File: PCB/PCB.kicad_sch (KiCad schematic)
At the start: 17 parts, among them J1 Conn_01x06_Pin, U2 A7106, U3 HT7333-3.3V, U4 STM32G031F6Px, Y1 16MHz

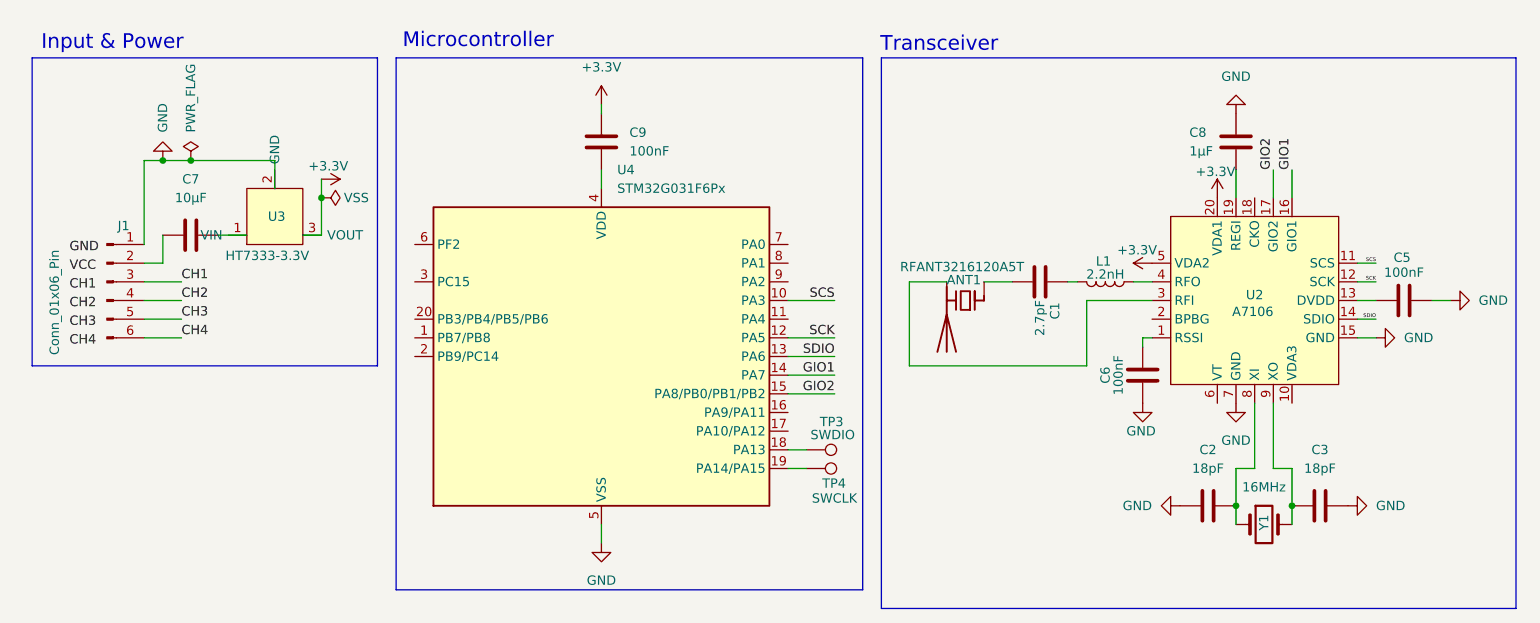
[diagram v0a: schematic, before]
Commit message: Wiring fixes
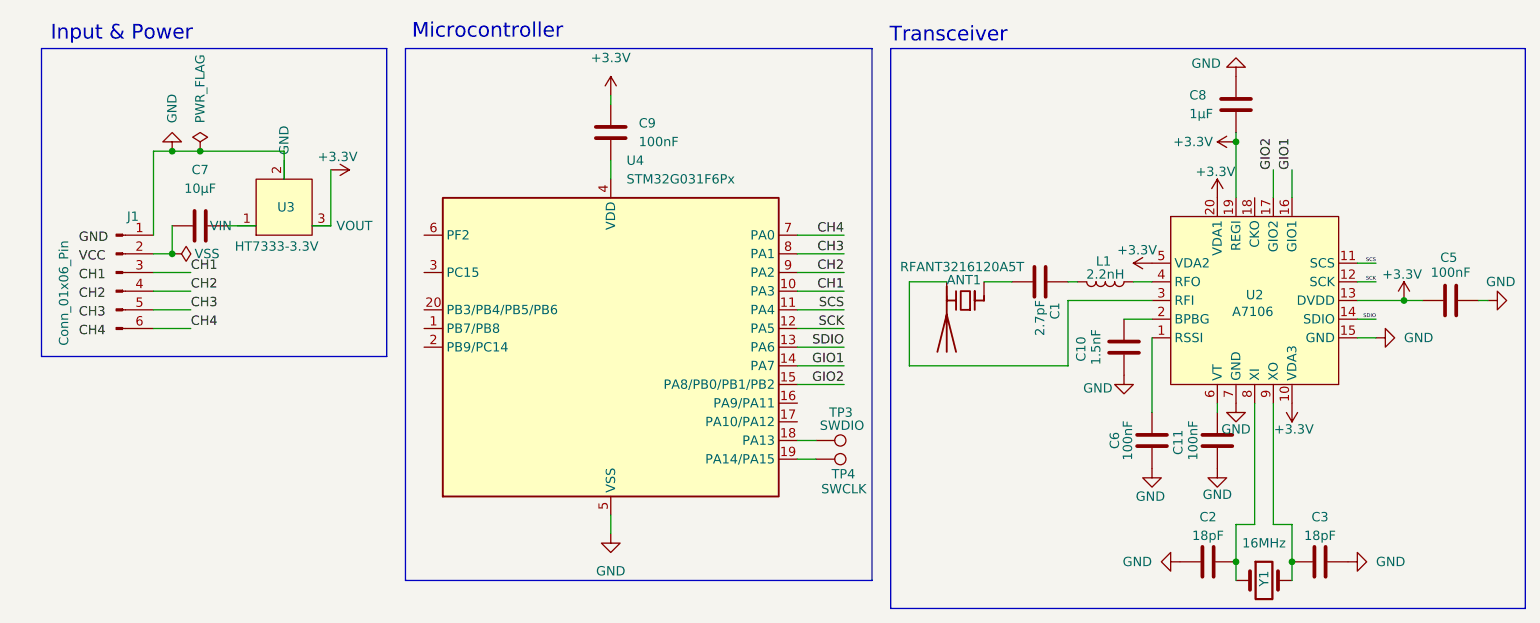
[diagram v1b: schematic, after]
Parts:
- added C10: 1.5nF, Capacitor_SMD:C_0402_1005Metric, symbol Device:C
- added C11: 100nF, Capacitor_SMD:C_0402_1005Metric, symbol Device:C
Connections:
- net +3.3V: now also C5.2, C8.2, U2.10 (VDA3), U2.13 (DVDD), U2.19 (REGI)
- net CH1: now also U4.10 (PA3)
- net CH2: now also U4.9 (PA2)
- net CH3: now also U4.8 (PA1)
- net CH4: now also U4.7 (PA0)
- net GND: now also C10.2, C11.2
- net SCS: now also U4.11 (PA4); no longer U4.10 (PA3)
- net at U2.2 (BPBG): now also C10.1
- net at U2.6 (VT): now also C11.1
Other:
- moved on the sheet: C2, C3, C5, C6, C7, C8, C9, J1, TP3, TP4, U3, U4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
